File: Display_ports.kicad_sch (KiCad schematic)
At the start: 9 parts, among them J2 DP_A

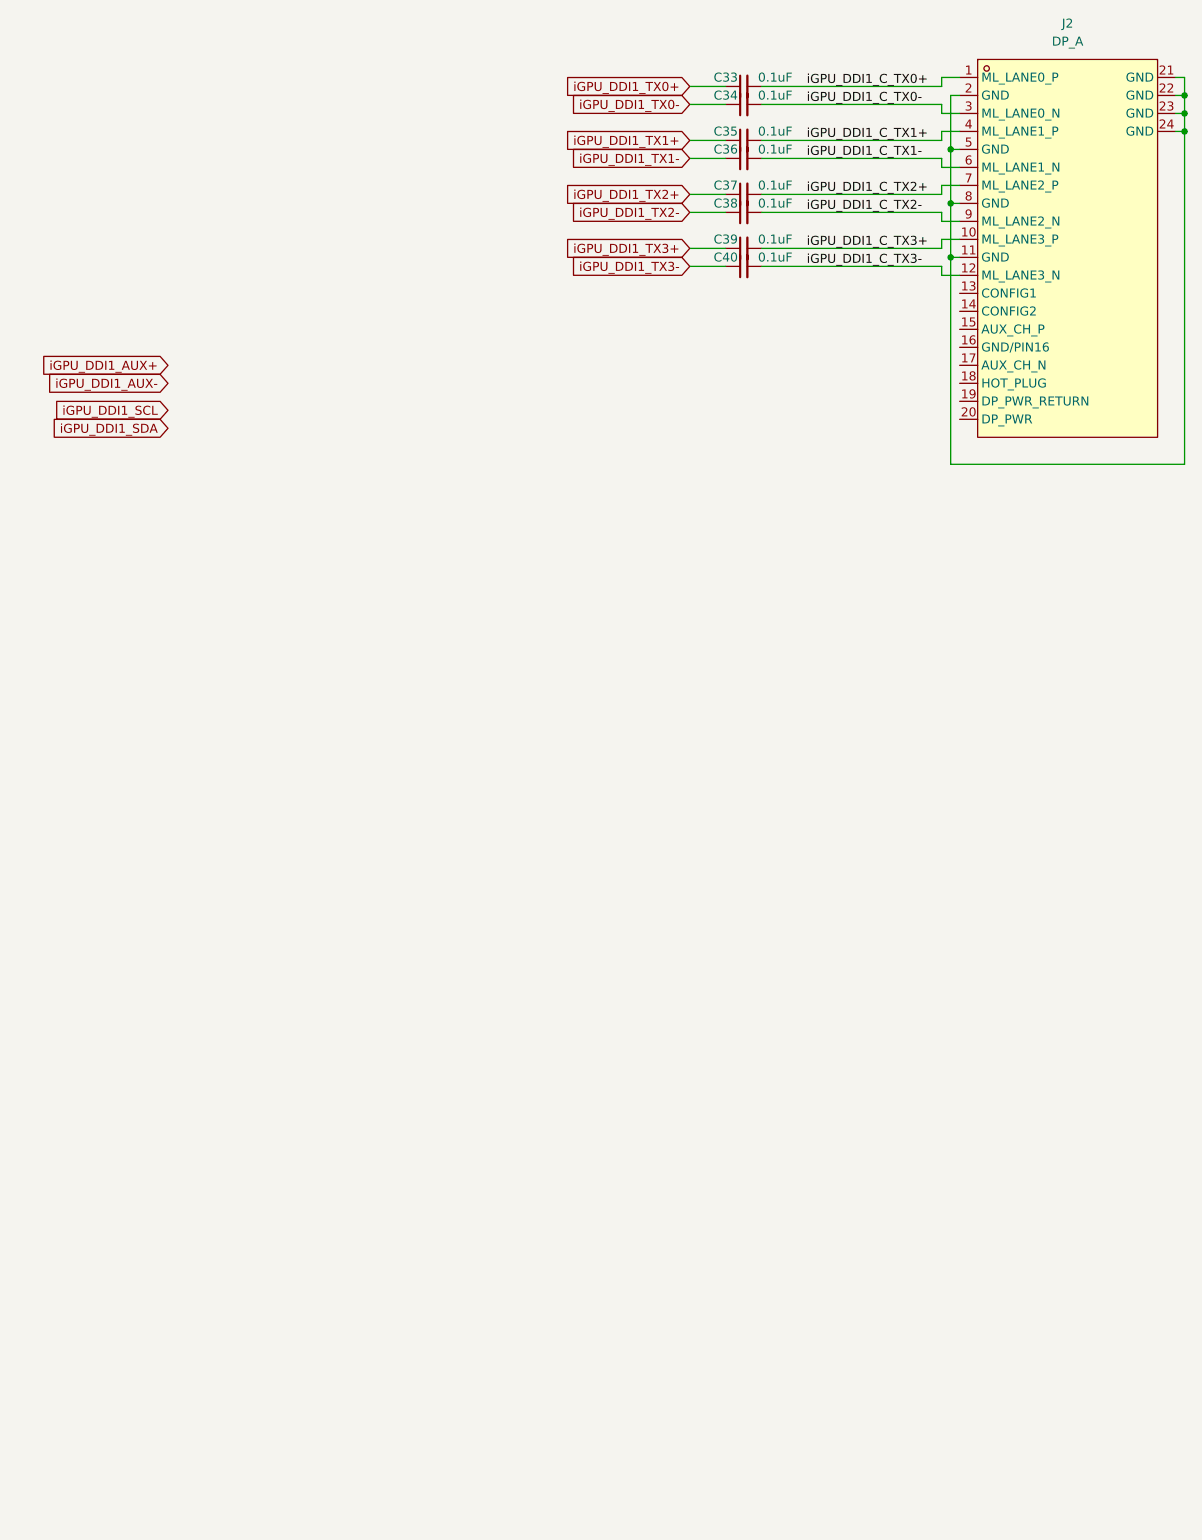
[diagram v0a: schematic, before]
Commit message: More DP
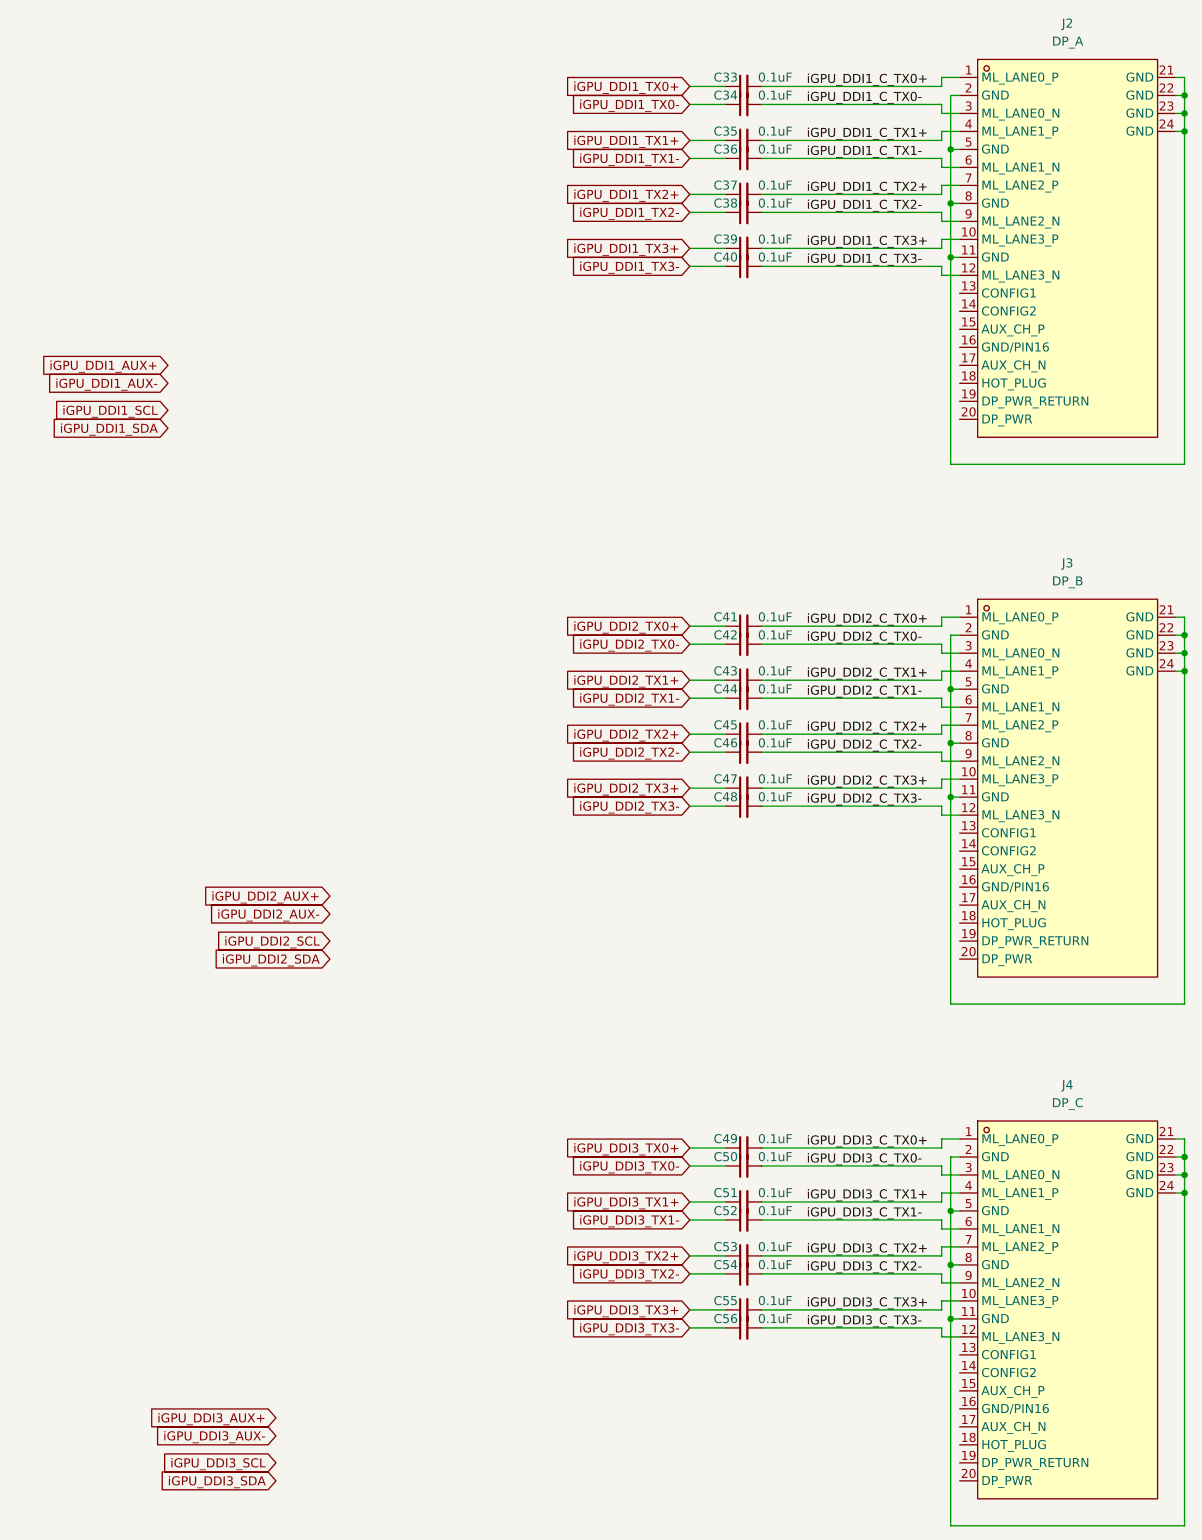
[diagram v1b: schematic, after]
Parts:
- added C41, C42, C43, C44, C45, C46, C47, C48, C49, C50, C51, C52, C53, C54, C55, C56: 0.1uF, Capacitor_SMD:C_0402_1005Metric, symbol Device:C_Small
- added J3: DP_B, A-my-stuff:DP-SMD_HYC16-DP20-178, symbol A-my-stuff:HYC16-DP20-178
- added J4: DP_C, A-my-stuff:DP-SMD_HYC16-DP20-178, symbol A-my-stuff:HYC16-DP20-178
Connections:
- new net: J3.11 (GND), J3.2 (GND), J3.21 (GND), J3.22 (GND), J3.23 (GND), J3.24 (GND), J3.5 (GND), J3.8 (GND)
- new net: J4.11 (GND), J4.2 (GND), J4.21 (GND), J4.22 (GND), J4.23 (GND), J4.24 (GND), J4.5 (GND), J4.8 (GND)
- new net iGPU_DDI2_C_TX0+: C41.2, J3.1 (ML_LANE0_P)
- new net iGPU_DDI2_C_TX0-: C42.2, J3.3 (ML_LANE0_N)
- new net iGPU_DDI2_C_TX1+: C43.2, J3.4 (ML_LANE1_P)
- new net iGPU_DDI2_C_TX1-: C44.2, J3.6 (ML_LANE1_N)
- new net iGPU_DDI2_C_TX2+: C45.2, J3.7 (ML_LANE2_P)
- new net iGPU_DDI2_C_TX2-: C46.2, J3.9 (ML_LANE2_N)
- new net iGPU_DDI2_C_TX3+: C47.2, J3.10 (ML_LANE3_P)
- new net iGPU_DDI2_C_TX3-: C48.2, J3.12 (ML_LANE3_N)
- new net iGPU_DDI2_TX0+: C41.1
- new net iGPU_DDI2_TX0-: C42.1
- new net iGPU_DDI2_TX1+: C43.1
- new net iGPU_DDI2_TX1-: C44.1
- new net iGPU_DDI2_TX2+: C45.1
- new net iGPU_DDI2_TX2-: C46.1
- new net iGPU_DDI2_TX3+: C47.1
- new net iGPU_DDI2_TX3-: C48.1
- new net iGPU_DDI3_C_TX0+: C49.2, J4.1 (ML_LANE0_P)
- new net iGPU_DDI3_C_TX0-: C50.2, J4.3 (ML_LANE0_N)
- new net iGPU_DDI3_C_TX1+: C51.2, J4.4 (ML_LANE1_P)
- new net iGPU_DDI3_C_TX1-: C52.2, J4.6 (ML_LANE1_N)
- new net iGPU_DDI3_C_TX2+: C53.2, J4.7 (ML_LANE2_P)
- new net iGPU_DDI3_C_TX2-: C54.2, J4.9 (ML_LANE2_N)
- new net iGPU_DDI3_C_TX3+: C55.2, J4.10 (ML_LANE3_P)
- new net iGPU_DDI3_C_TX3-: C56.2, J4.12 (ML_LANE3_N)
- new net iGPU_DDI3_TX0+: C49.1
- new net iGPU_DDI3_TX0-: C50.1
- new net iGPU_DDI3_TX1+: C51.1
- new net iGPU_DDI3_TX1-: C52.1
- new net iGPU_DDI3_TX2+: C53.1
- new net iGPU_DDI3_TX2-: C54.1
- new net iGPU_DDI3_TX3+: C55.1
- new net iGPU_DDI3_TX3-: C56.1
